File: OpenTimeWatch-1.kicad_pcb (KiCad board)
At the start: 2 copper layers, 1 part

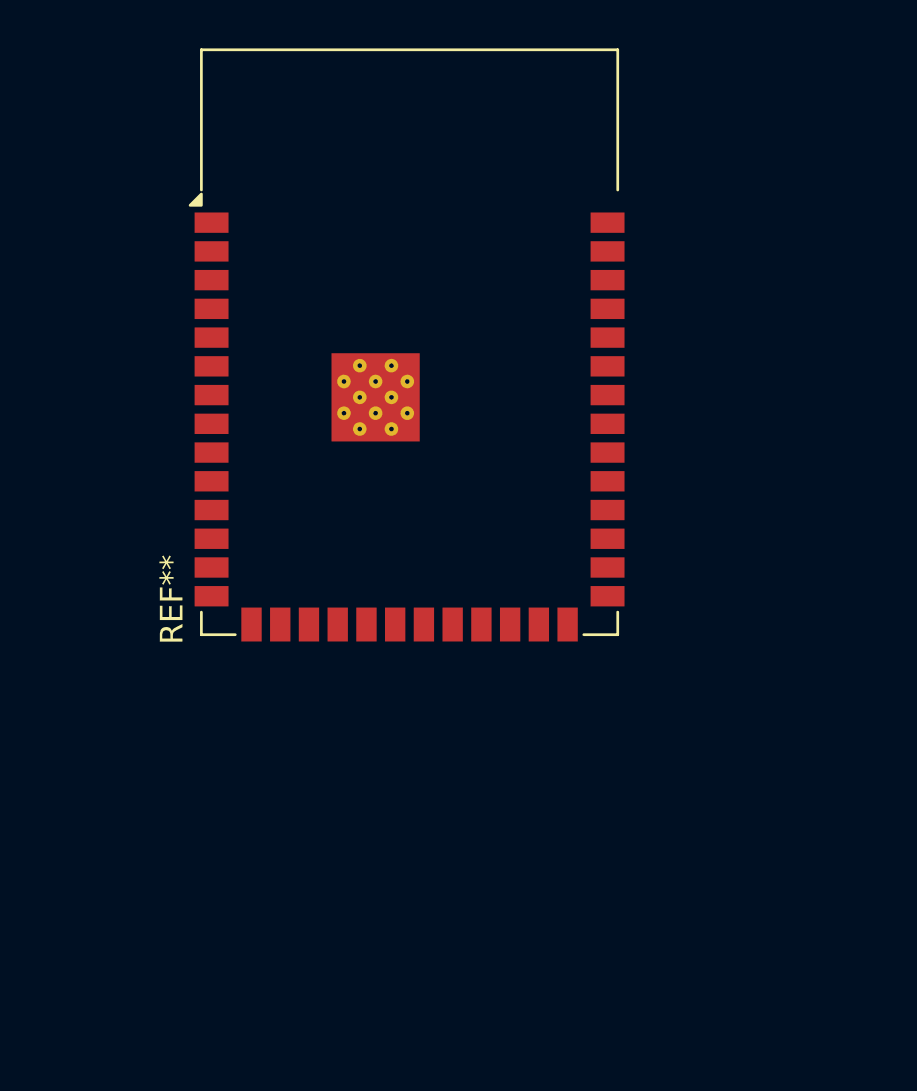
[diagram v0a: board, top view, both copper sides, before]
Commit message: Update PCB schematics and design files
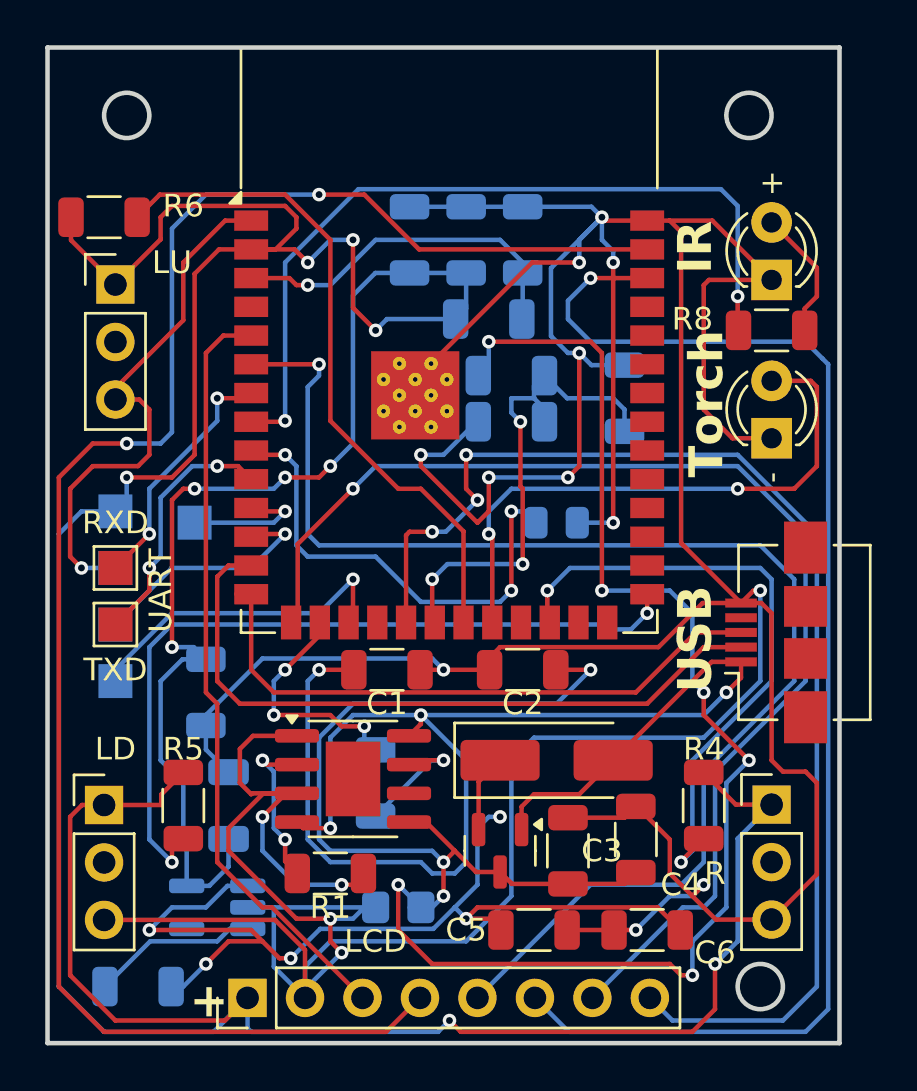
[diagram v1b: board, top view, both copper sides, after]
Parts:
- added REF**: PinHeader_1x03_P2.54mm_Vertical, Connector_PinHeader_2.54mm:PinHeader_1x03_P2.54mm_Vertical, F.Cu at (121.0, 94.5)
- added REF**: LED_D3.0mm_IRBlack, LED_THT:LED_D3.0mm_IRBlack, F.Cu at (150.5, 71.3)
- added REF**: R_1206_3216Metric, Resistor_SMD:R_1206_3216Metric, F.Cu at (133.5, 88.5)
- added REF**: PinHeader_1x08_P2.54mm_Vertical, Connector_PinHeader_2.54mm:PinHeader_1x08_P2.54mm_Vertical, F.Cu at (127.3, 103.0)
- added REF**: LED_D3.0mm_IRBlack, LED_THT:LED_D3.0mm_IRBlack, F.Cu at (150.5, 78.3)
- added REF**: USB_Micro-B_Amphenol_10104110_Horizontal, Connector_USB:USB_Micro-B_Amphenol_10104110_Horizontal, F.Cu at (150.7, 86.8)
- added REF**: R_1206_3216Metric, Resistor_SMD:R_1206_3216Metric, F.Cu at (145.0, 100.0)
- added REF**: R_1206_3216Metric, Resistor_SMD:R_1206_3216Metric, F.Cu at (131.0, 97.5)
- added REF**: TestPoint_Pad_1.5x1.5mm, TestPoint:TestPoint_Pad_1.5x1.5mm, F.Cu at (121.5, 86.5)
- added REF**: SOT-23, Package_TO_SOT_SMD:SOT-23, F.Cu at (138.5, 96.5)
- added REF**: D_SMA_Handsoldering, Diode_SMD:D_SMA_Handsoldering, F.Cu at (141.0, 92.5)
- added REF**: R_1206_3216Metric, Resistor_SMD:R_1206_3216Metric, F.Cu at (147.5, 94.5)
- added REF**: PinHeader_1x03_P2.54mm_Vertical, Connector_PinHeader_2.54mm:PinHeader_1x03_P2.54mm_Vertical, F.Cu at (150.5, 94.5)
- added REF**: SOIC-8-1EP_3.9x4.9mm_P1.27mm_EP2.41x3.3mm, Package_SO:SOIC-8-1EP_3.9x4.9mm_P1.27mm_EP2.41x3.3mm, F.Cu at (132.0, 93.3)
- added REF**: R_1206_3216Metric, Resistor_SMD:R_1206_3216Metric, F.Cu at (121.0, 68.5)
- added REF**: TestPoint_Pad_1.5x1.5mm, TestPoint:TestPoint_Pad_1.5x1.5mm, F.Cu at (121.5, 84.0)
- added REF**: TestPoint_Pad_1.5x1.5mm, TestPoint:TestPoint_Pad_1.5x1.5mm, B.Cu at (121.5, 84.0)
- added REF**: SOT-23-5_HandSoldering, Package_TO_SOT_SMD:SOT-23-5_HandSoldering, B.Cu at (126.0, 99.0)
- added REF**: R_1206_3216Metric, Resistor_SMD:R_1206_3216Metric, B.Cu at (139.0, 75.5)
- added REF**: R_1206_3216Metric, Resistor_SMD:R_1206_3216Metric, B.Cu at (144.0, 76.5)
- added REF**: TestPoint_Pad_1.5x1.5mm, TestPoint:TestPoint_Pad_1.5x1.5mm, B.Cu at (121.5, 81.5)
- added REF**: R_1206_3216Metric, Resistor_SMD:R_1206_3216Metric, F.Cu at (141.5, 96.5)
- added REF**: R_1206_3216Metric, Resistor_SMD:R_1206_3216Metric, B.Cu at (134.5, 69.5)
- added REF**: R_1206_3216Metric, Resistor_SMD:R_1206_3216Metric, B.Cu at (137.0, 69.5)
- added REF**: TestPoint_Pad_1.5x1.5mm, TestPoint:TestPoint_Pad_1.5x1.5mm, B.Cu at (121.5, 86.5)
- added REF**: R_1206_3216Metric, Resistor_SMD:R_1206_3216Metric, B.Cu at (139.0, 77.5)
- added REF**: R_0805_2012Metric_Pad1.20x1.40mm_HandSolder, Resistor_SMD:R_0805_2012Metric_Pad1.20x1.40mm_HandSolder, B.Cu at (134.0, 99.0)
- added REF**: R_1206_3216Metric, Resistor_SMD:R_1206_3216Metric, B.Cu at (138.0, 73.0)
- added REF**: R_1206_3216Metric, Resistor_SMD:R_1206_3216Metric, B.Cu at (125.5, 89.5)
- added REF**: TestPoint_Pad_1.5x1.5mm, TestPoint:TestPoint_Pad_1.5x1.5mm, B.Cu at (125.0, 82.0)
- added REF**: R_1206_3216Metric, Resistor_SMD:R_1206_3216Metric, B.Cu at (122.5, 102.5)
- added REF**: R_1206_3216Metric, Resistor_SMD:R_1206_3216Metric, B.Cu at (139.5, 69.5)
- added REF**: R_1206_3216Metric, Resistor_SMD:R_1206_3216Metric, F.Cu at (144.5, 96.0)
- added REF**: R_1206_3216Metric, Resistor_SMD:R_1206_3216Metric, B.Cu at (133.0, 93.5)
- added REF**: TestPoint_Pad_1.5x1.5mm, TestPoint:TestPoint_Pad_1.5x1.5mm, B.Cu at (121.5, 89.0)
- added REF**: R_0805_2012Metric, Resistor_SMD:R_0805_2012Metric, B.Cu at (141.0, 82.0)
- added REF**: C_1206_3216Metric, Capacitor_SMD:C_1206_3216Metric, B.Cu at (126.5, 94.5)
- added REF**: R_1206_3216Metric, Resistor_SMD:R_1206_3216Metric, F.Cu at (150.5, 73.5)
- added REF**: R_1206_3216Metric, Resistor_SMD:R_1206_3216Metric, F.Cu at (124.5, 94.5)
- added REF**: R_1206_3216Metric, Resistor_SMD:R_1206_3216Metric, F.Cu at (140.0, 100.0)
- added REF**: R_1206_3216Metric, Resistor_SMD:R_1206_3216Metric, F.Cu at (139.5, 88.5)
- added REF**: PinHeader_1x03_P2.54mm_Vertical, Connector_PinHeader_2.54mm:PinHeader_1x03_P2.54mm_Vertical, F.Cu at (121.5, 71.5)
- moved REF** 1.75 mm to (136.2, 73.9)
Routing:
- net (no net): track 0.00 -> 1377.6 mm, vias 0 -> 81
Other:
- board outline added: 35 x 44 mm
- board text added: "+"
- board text added: "+ -"
- board text added: "-"
- board text added: "- +"
- board text added: "Accel"
- board text added: "BAT"
- board text added: "C1"
- board text added: "C10"
- board text added: "C11"
- board text added: "C12"
- board text added: "C2"
- board text added: "C3"
- board text added: "C4"
- board text added: "C5"
- board text added: "C6"
- board text added: "C7"
- board text added: "C8"
- board text added: "C9"
- board text added: "Heart"
- board text added: "IR"
- board text added: "LCD"
- board text added: "LD"
- board text added: "LU"
- board text added: "Made by Jaswanth Venkata Sai Chennu"
- board text added: "OpenTimeWatch 1"
- board text added: "R"
- board text added: "R1"
- board text added: "R10"
- board text added: "R11"
- board text added: "R2"
- board text added: "R3"
- board text added: "R4"
- board text added: "R5"
- board text added: "R6"
- board text added: "R8"
- board text added: "R9"
- board text added: "RXD"
- board text added: "SPKR"
- board text added: "TXD"
- board text added: "Torch"
- board text added: "UART"
- board text added: "USB"
